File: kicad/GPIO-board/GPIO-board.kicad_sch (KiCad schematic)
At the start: 29 parts, among them J19 Conn_01x02, J20 BANANA JACK HV, J21 Conn_01x04, J22 Conn_01x02, J23 BANANA JACK LV, J24 Conn_02x15_Top_Bottom, U14 MP2307

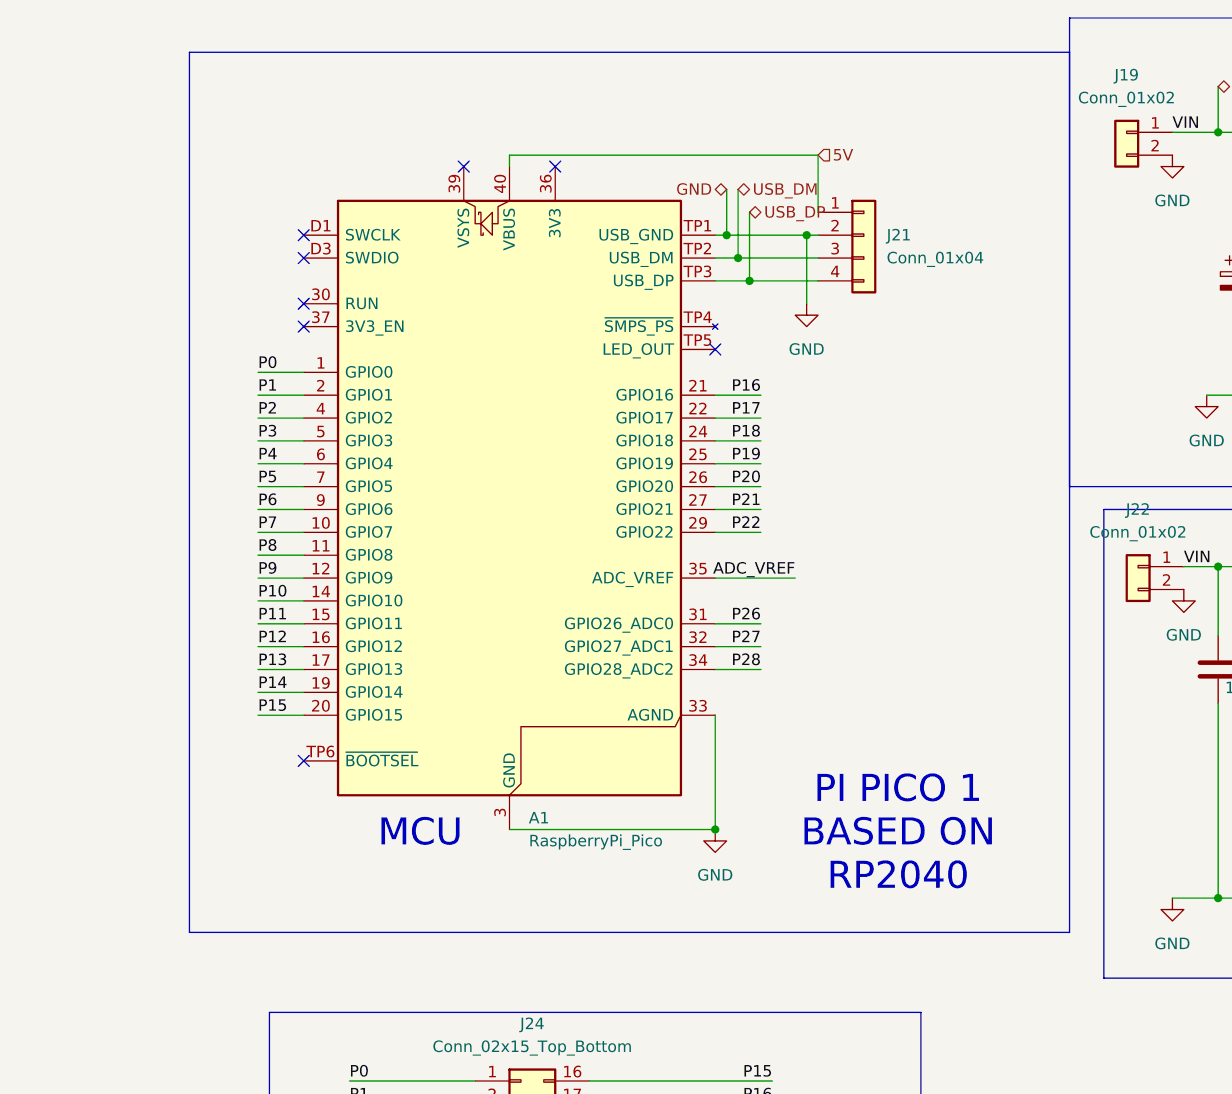
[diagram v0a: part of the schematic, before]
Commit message: DOCUMENTED Till the Navigation board
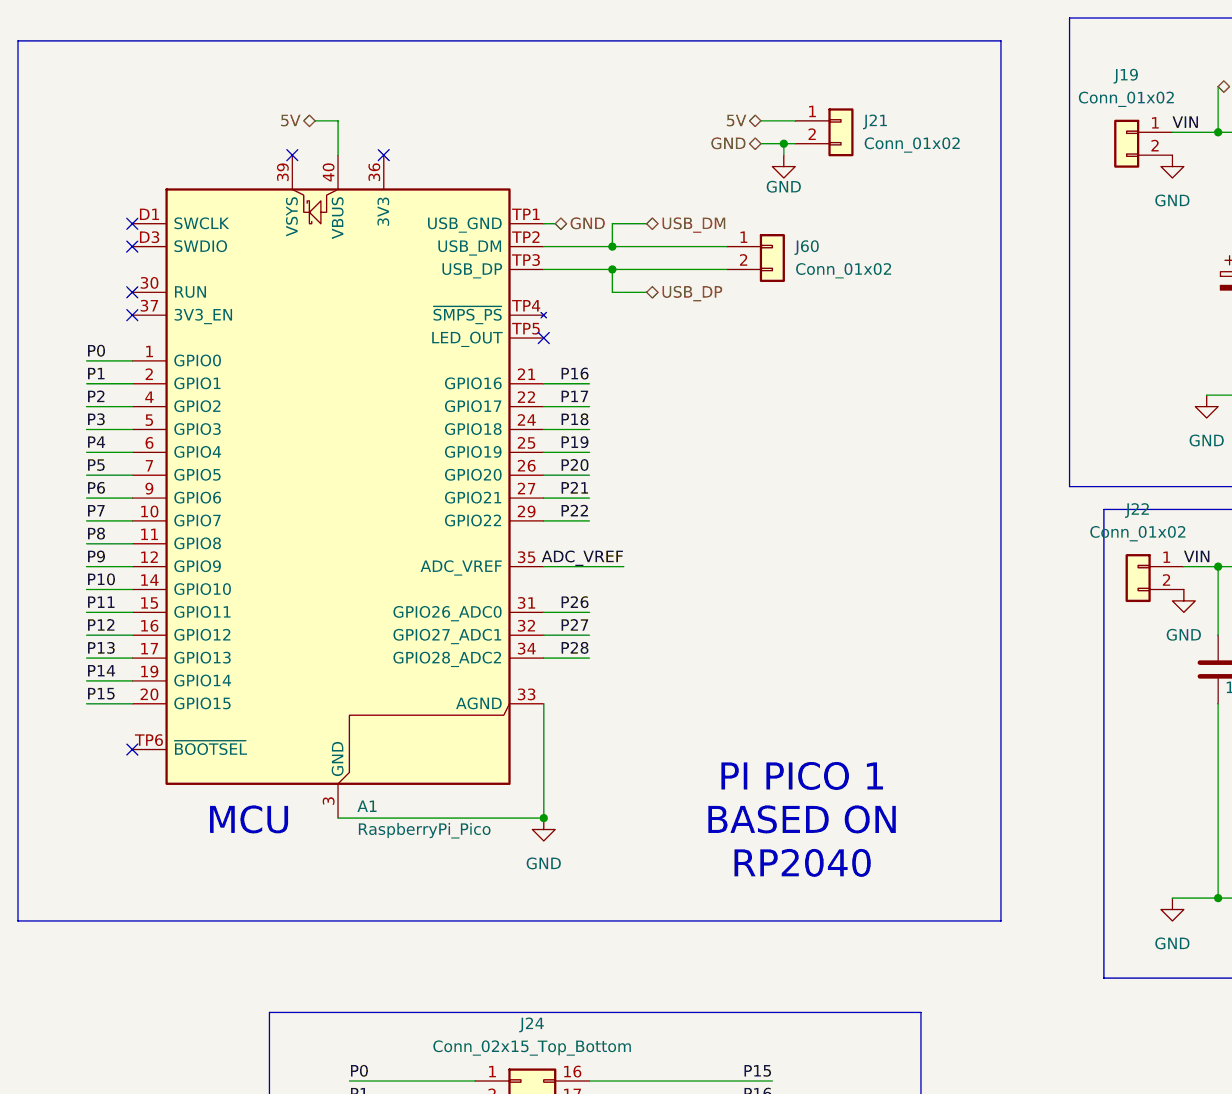
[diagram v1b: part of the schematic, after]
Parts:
- removed J21: Conn_01x04, symbol Connector_Generic:Conn_01x04
- added J21, J60: Conn_01x02, symbol Connector_Generic:Conn_01x02
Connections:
- net 5V: now also J21.1 (Pin_1)
- net GND: now also J21.2 (Pin_2)
- net USB_DM: now also J60.1 (Pin_1)
- net USB_DP: now also J60.2 (Pin_2)
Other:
- moved on the sheet: A1
